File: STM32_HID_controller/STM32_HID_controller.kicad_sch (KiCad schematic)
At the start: 49 parts, among them J1 USB_B_Micro, J2 Conn_01x04_Pin, J3 Conn_01x03_Pin, J5 Conn_01x03_Pin, SW1 SW_SPDT, SW10 SW_Push, SW11 SW_Push, SW14 SW_Push, SW2 SW_Push, SW3 SW_Push, SW6 SW_Push, SW7 SW_Push, SW8 SW_Push, SW9 SW_Push, U1 STM32F446RETx, U2 AMS1117-3.3, U3 ADXL345, U4 joystick_right, U5 joystick_left, Y1 8MHz

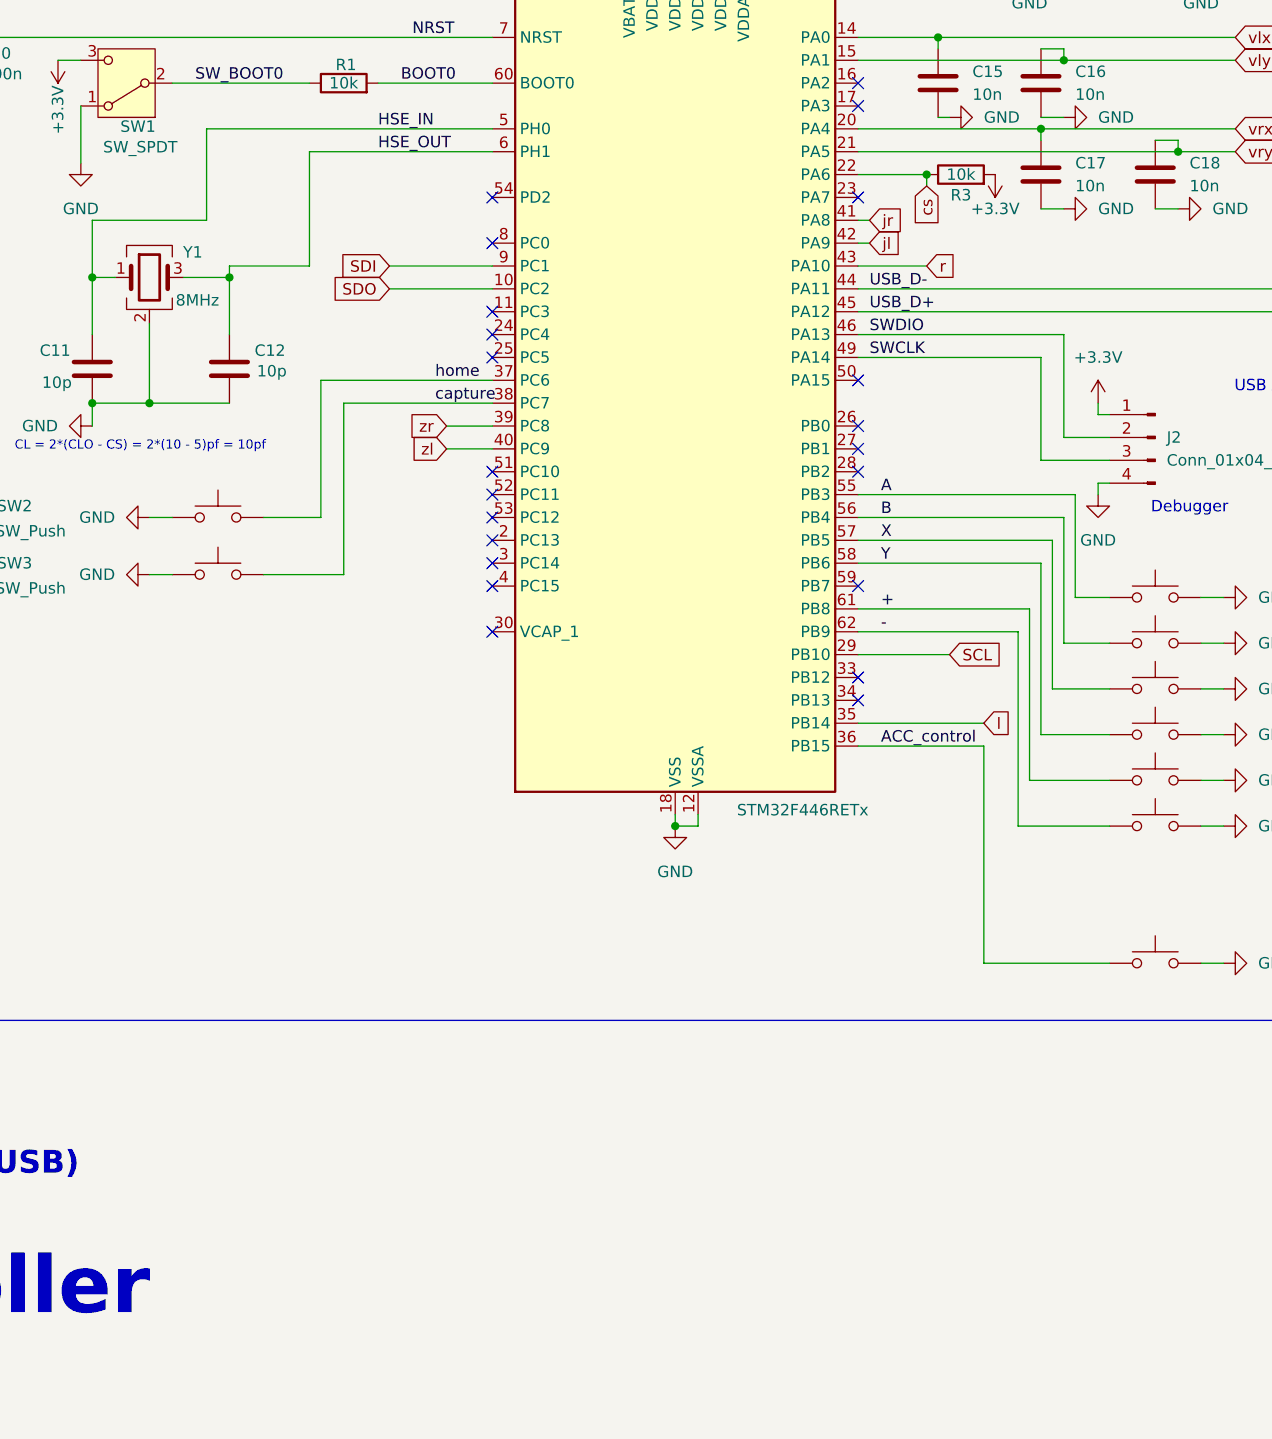
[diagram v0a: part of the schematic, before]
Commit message: Started flux for left and right
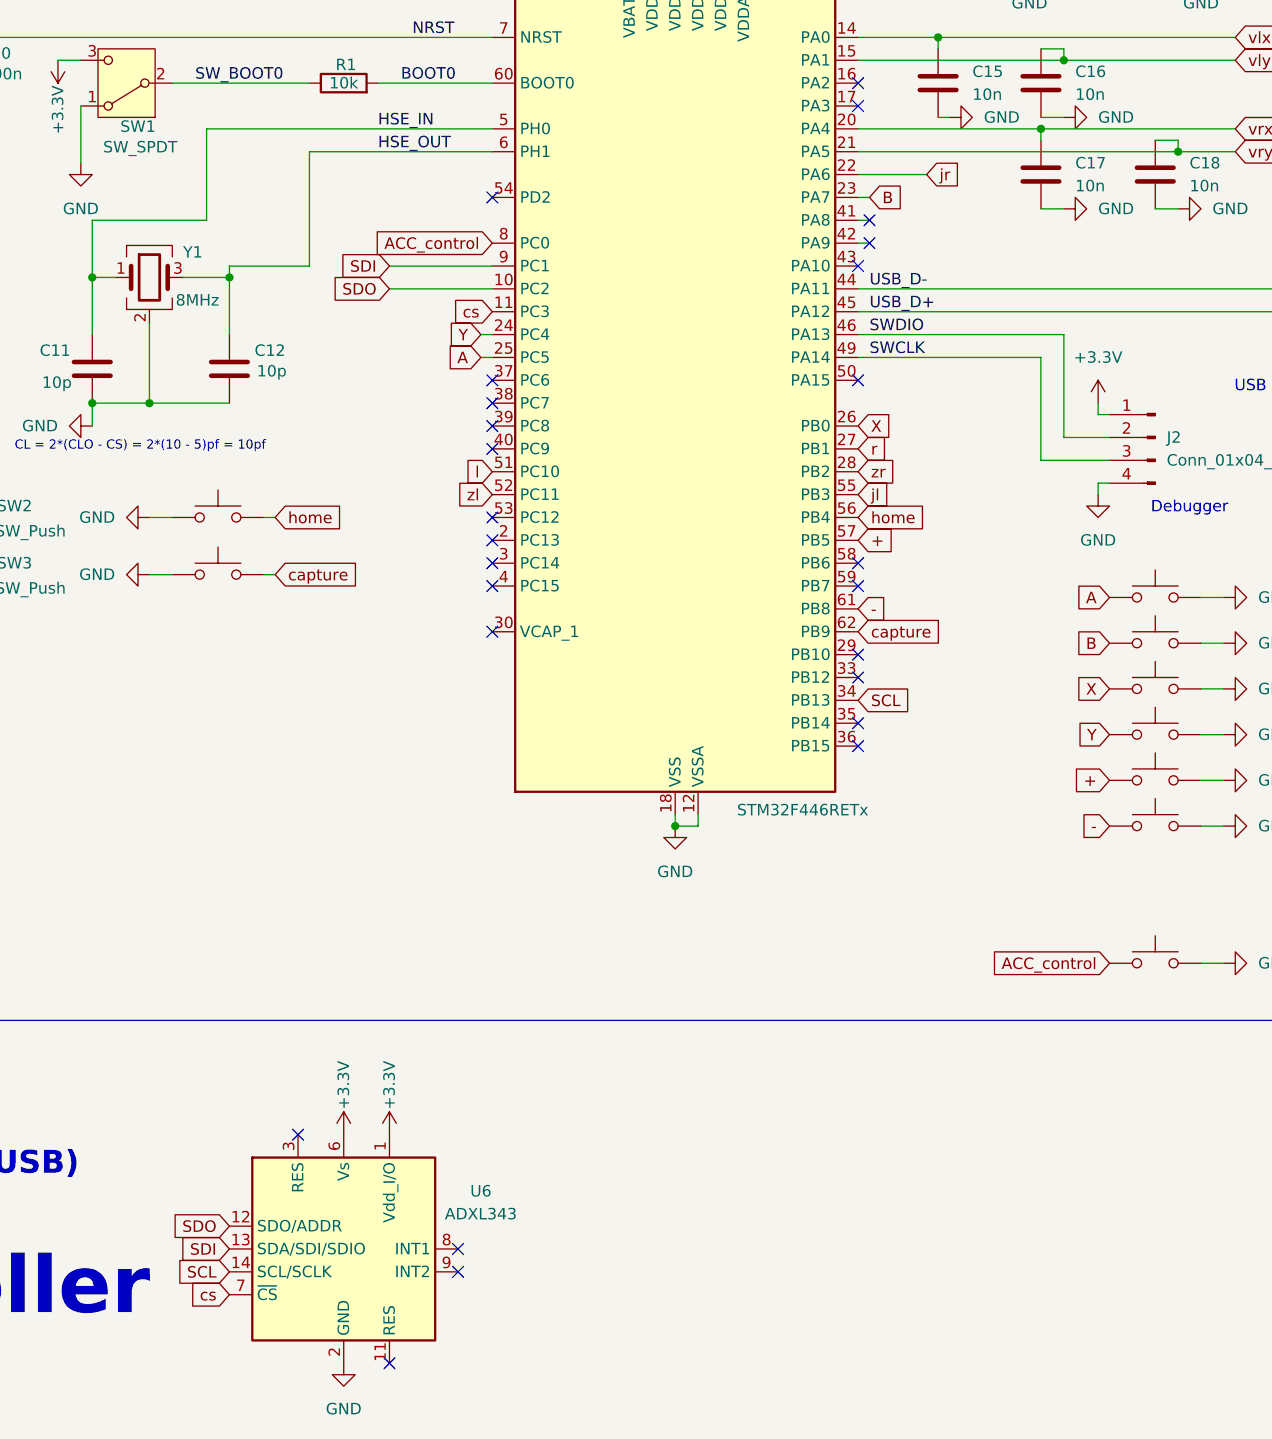
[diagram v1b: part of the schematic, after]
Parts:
- removed R3: 10k, Resistor_SMD:R_0402_1005Metric, symbol Device:R
- added U6: ADXL343, Package_LGA:LGA-14_3x5mm_P0.8mm_LayoutBorder1x6y, symbol Sensor_Motion:ADXL343
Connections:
- net +: now also U1.57 (PB5); no longer U1.61 (PB8)
- net +3.3V: now also U6.1 (Vdd_I/O), U6.6 (Vs)
- net -: now also U1.61 (PB8); no longer U1.62 (PB9)
- net A: now also U1.25 (PC5); no longer U1.55 (PB3)
- net ACC_control: now also U1.8 (PC0); no longer U1.36 (PB15)
- net B: now also U1.23 (PA7); no longer U1.56 (PB4)
- net GND: now also U6.2 (GND), U6.4 (GND), U6.5 (GND)
- net SCL: now also U1.34 (PB13), U6.14 (SCL/SCLK); no longer U1.29 (PB10)
- net SDI: now also U6.13 (SDA/SDI/SDIO)
- net SDO: now also U6.12 (SDO/ADDR)
- net X: now also U1.26 (PB0); no longer U1.57 (PB5)
- net Y: now also U1.24 (PC4); no longer U1.58 (PB6)
- net capture: now also U1.62 (PB9); no longer U1.38 (PC7)
- net cs: now also U1.11 (PC3), U6.7 (~{CS}); no longer U1.22 (PA6)
- net home: now also U1.56 (PB4); no longer U1.37 (PC6)
- net jl: now also U1.55 (PB3); no longer U1.42 (PA9)
- net jr: now also U1.22 (PA6); no longer U1.41 (PA8)
- net l: now also U1.51 (PC10); no longer U1.35 (PB14)
- net r: now also U1.27 (PB1); no longer U1.43 (PA10)
- net zl: now also U1.52 (PC11); no longer U1.40 (PC9)
- net zr: now also U1.28 (PB2); no longer U1.39 (PC8)
- no-connect marks 29 -> 33
